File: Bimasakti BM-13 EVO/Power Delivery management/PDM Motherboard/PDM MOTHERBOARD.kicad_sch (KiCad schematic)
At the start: 24 parts

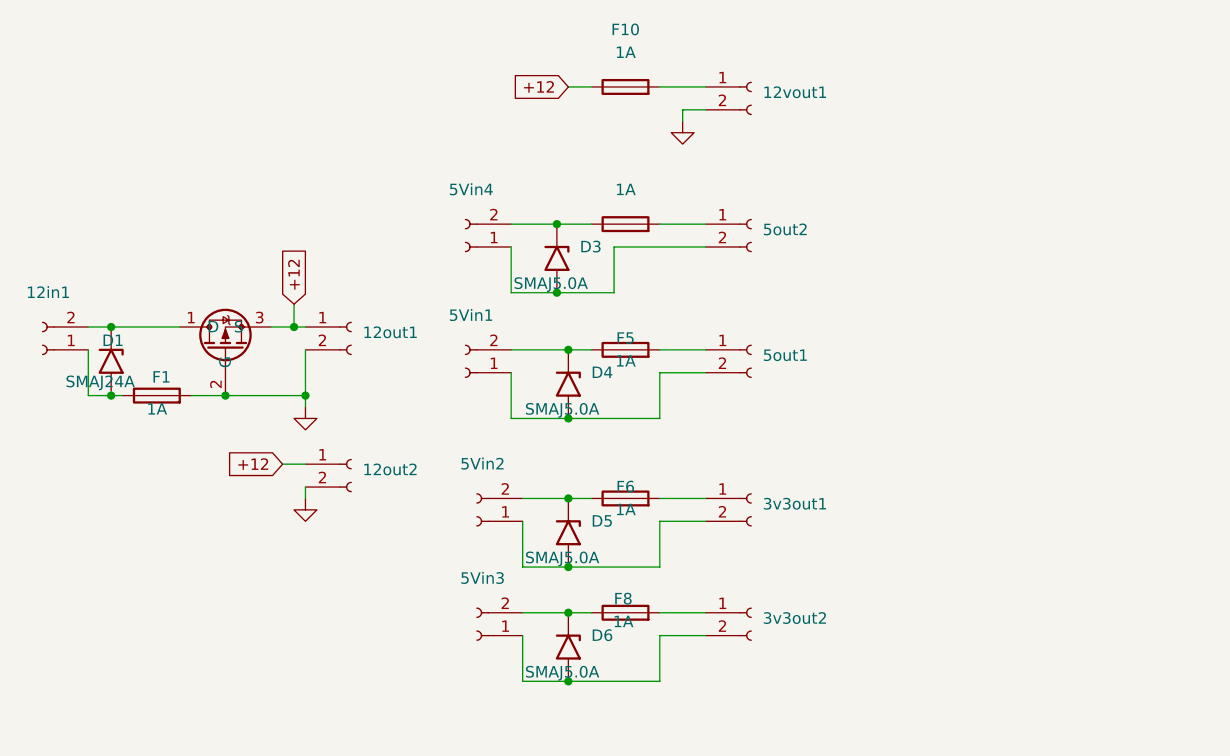
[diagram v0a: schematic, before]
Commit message: update motherboard pdm selesai
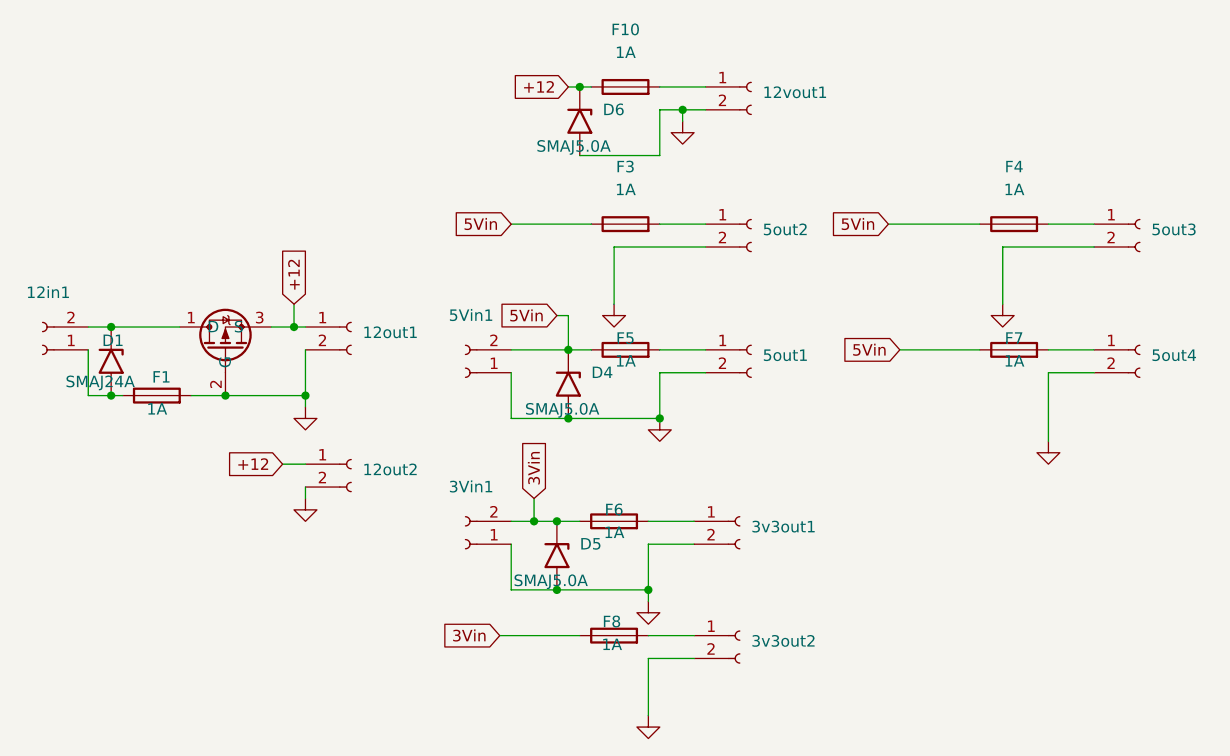
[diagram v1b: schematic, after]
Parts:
- removed 5Vin3, 5Vin4: ~, Connector_JST:JST_EH_B2B-EH-A_1x02_P2.50mm_Vertical, symbol Connector:Conn_01x02_Socket
- removed D3: SMAJ5.0A, Diode_SMD:D_SMA, symbol Diode:SMAJ5.0A
- added 5out3, 5out4: ~, Connector_JST:JST_EH_B2B-EH-A_1x02_P2.50mm_Vertical, symbol Connector:Conn_01x02_Socket
- added F4, F7: 1A, Fuse:Fuseholder_Cylinder-5x20mm_Schurter_0031_8201_Horizontal_Open, symbol Device:Fuse
- F1, F10, F3, F5, F6, F8: footprint Fuse:Fuseholder_Clip-5x20mm_Bel_FC-203-22_Lateral_P17.80x5.00mm_D1.17mm_Horizontal -> Fuse:Fuseholder_Cylinder-5x20mm_Schurter_0031_8201_Horizontal_Open
- U1: footprint Library:SOIC-8 (AOD) -> AO4407A:SOIC-8 (AOD)
- renumbered 5Vin2 to 3Vin1
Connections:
- net +12: now also D6.1 (A1)
- net GND: now also 3Vin1.1 (Pin_1), 3v3out1.2 (Pin_2), 3v3out2.2 (Pin_2), 5Vin1.1 (Pin_1), 5out1.2 (Pin_2), 5out2.2 (Pin_2), D4.2 (A2), D5.2 (A2), D6.2 (A2), 5out3.2 (Pin_2), 5out4.2 (Pin_2)
- net 3Vin: now reaches F8.1
- net 3Vin: now also 3Vin1.2 (Pin_2), D5.1 (A1), F6.1; no longer D6.1 (A1)
- net 5Vin: now reaches F3.1
- net 5Vin: now also 5Vin1.2 (Pin_2), D4.1 (A1), F5.1, F4.1, F7.1
- new net: 5out3.1 (Pin_1), F4.2
- new net: 5out4.1 (Pin_1), F7.2
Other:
- moved on the sheet: 3Vin1, 3v3out1, 3v3out2, D5, F6, F8
